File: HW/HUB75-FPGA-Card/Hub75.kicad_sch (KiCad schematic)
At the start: 12 parts, among them J1 Conn_02x08_Odd_Even, J2 Conn_02x08_Odd_Even, J3 Conn_01x03, J4 Conn_01x03, J5 Conn_01x03, J6 Conn_01x03, U2 74AHCT245PW, U3 74AHCT245PW, U4 74AHCT245PW

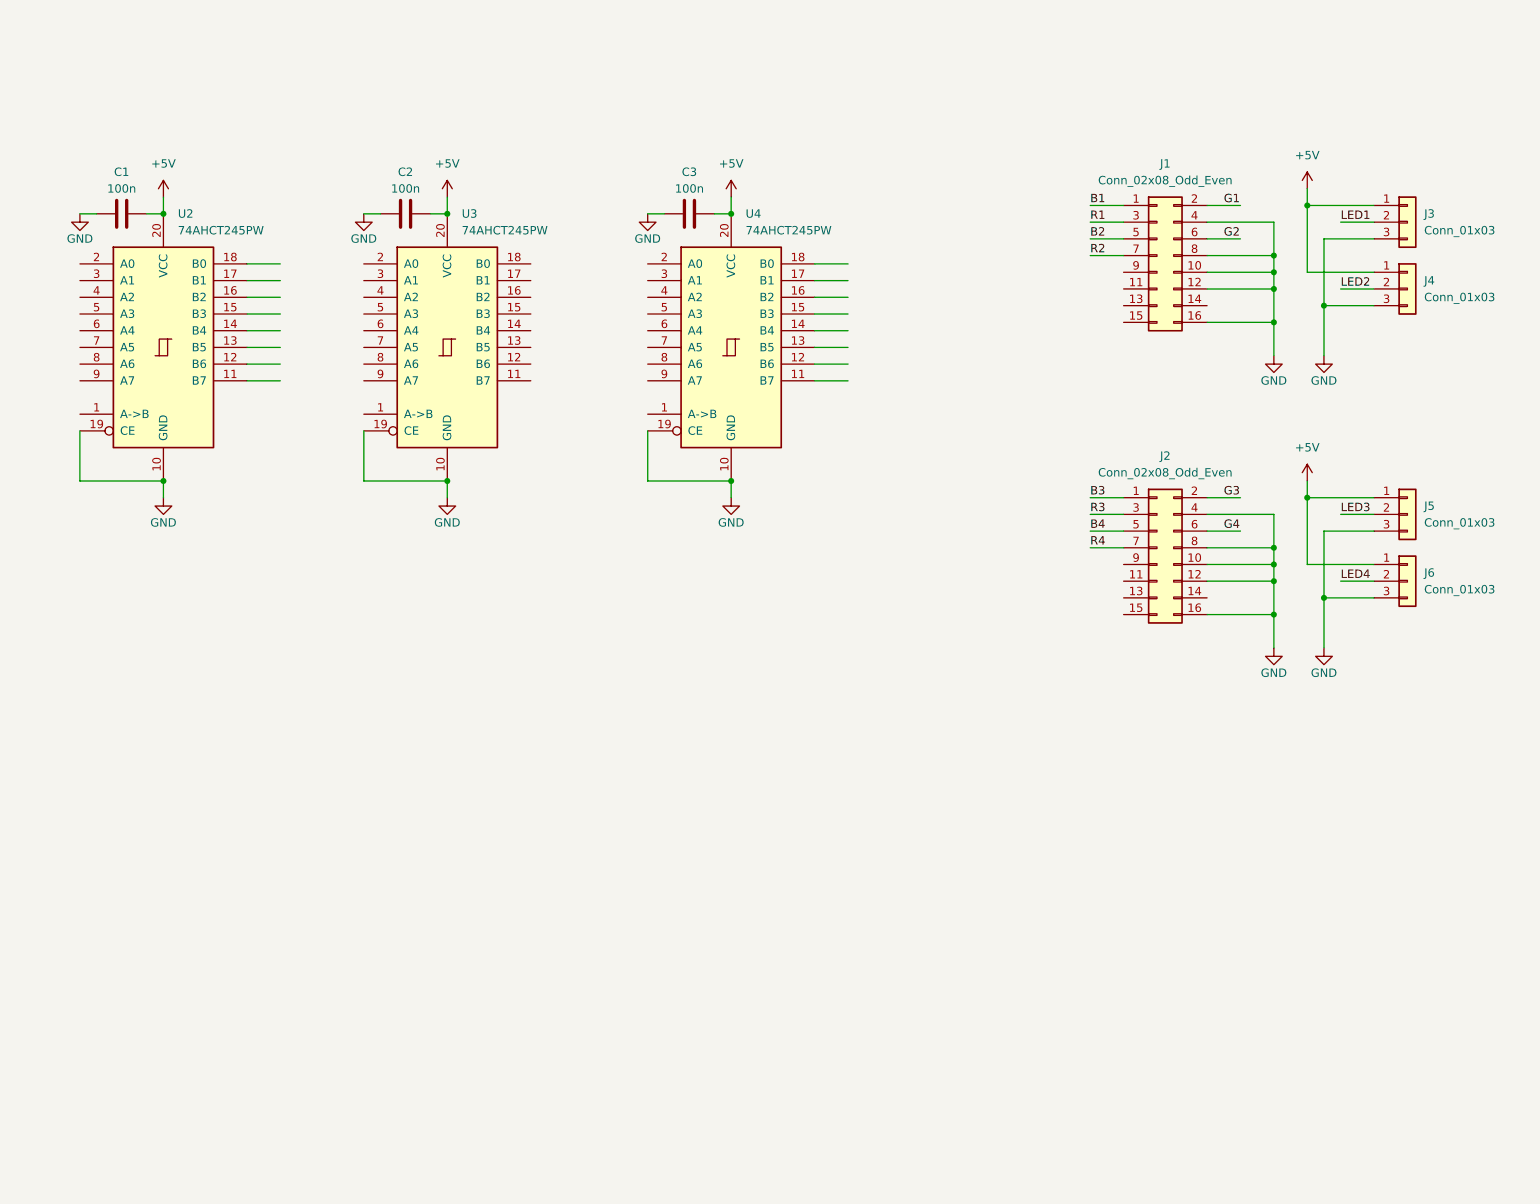
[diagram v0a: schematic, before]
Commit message: add usb audio implementation
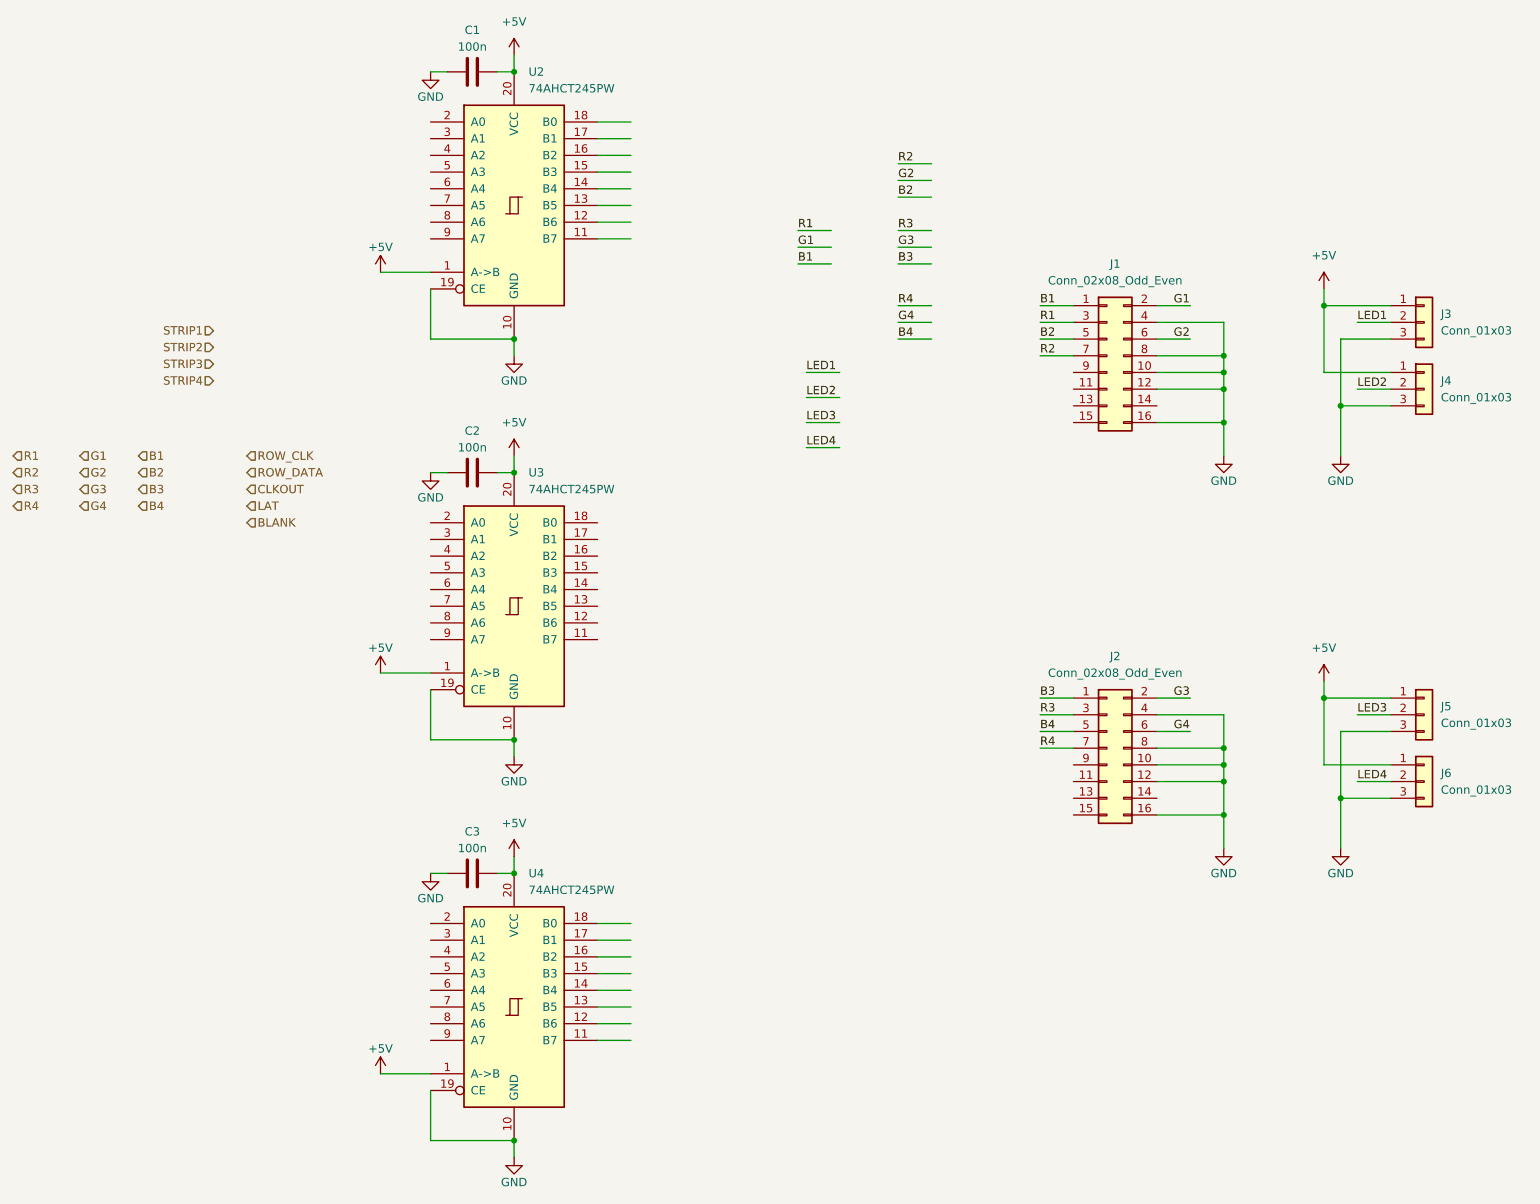
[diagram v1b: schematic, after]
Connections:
- net +5V: now also U2.1 (A->B), U3.1 (A->B), U4.1 (A->B)
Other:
- moved on the sheet: C1, C2, C3, J1, J2, J3, J4, J5, J6, U2, U3, U4
